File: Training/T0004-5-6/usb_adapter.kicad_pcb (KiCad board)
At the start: 2 copper layers, 50.8 x 25.4 mm, 23 parts, among them J1 modular8_rev3_comms_out, P1 USB_OTG, U1 FT231X, U2 TE_1825058-1

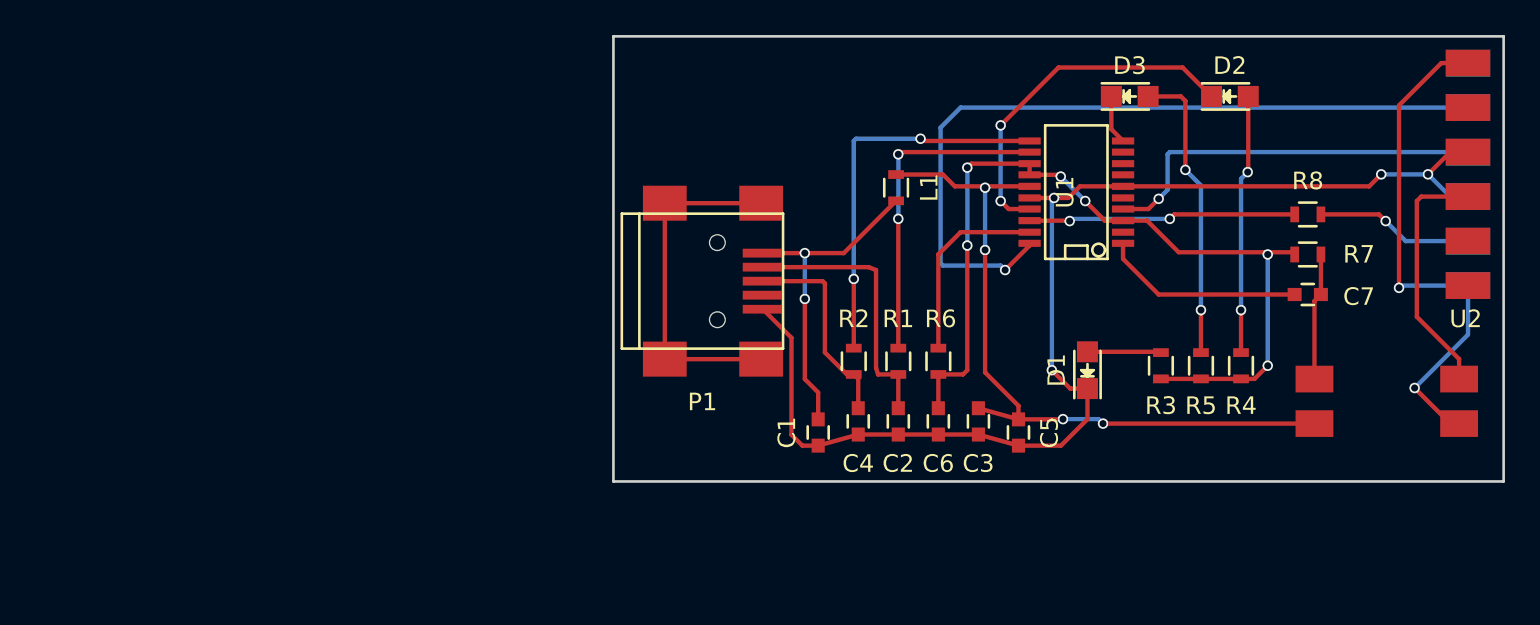
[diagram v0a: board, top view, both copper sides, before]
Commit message: generated gerbers
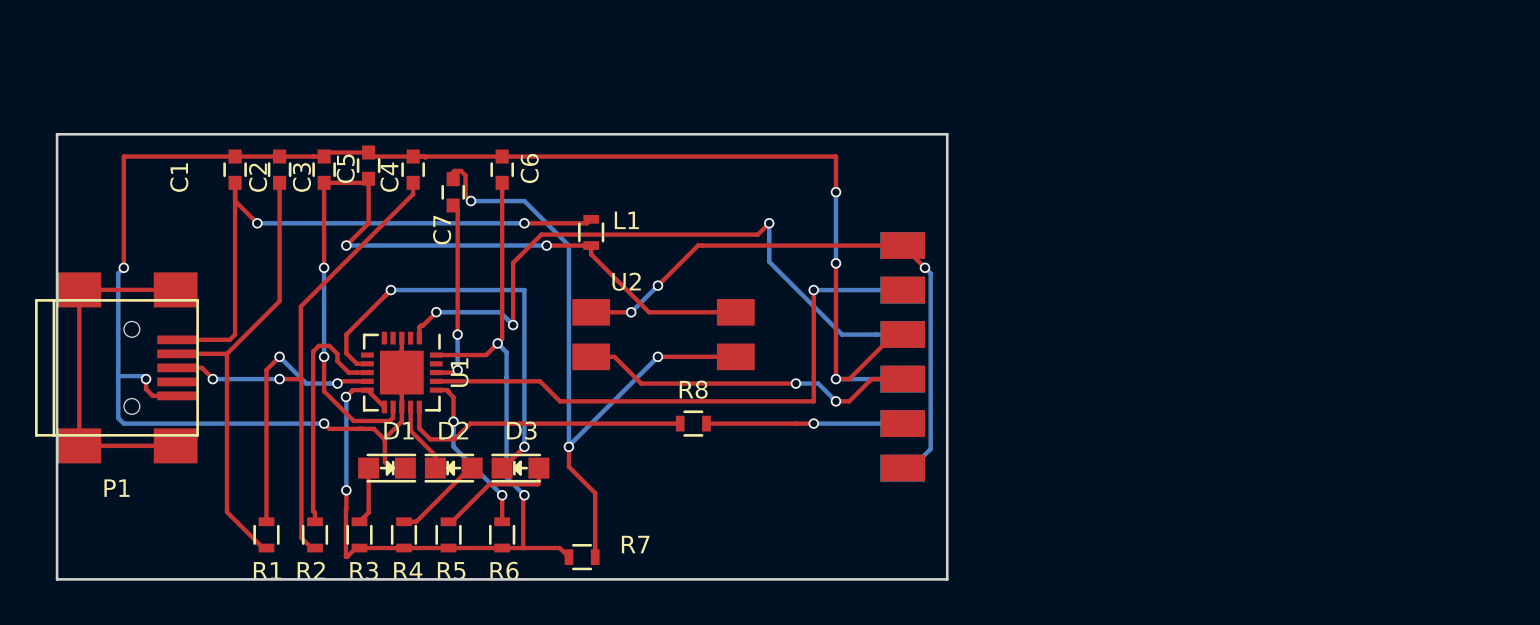
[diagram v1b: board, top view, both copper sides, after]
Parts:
- U1: value FT231X -> FT231XQ; footprint SMD_Packages:SSOP-20 -> Housings_DFN_QFN:QFN-20-1EP_4x4mm_Pitch0.5mm
- moved U2 49.9 mm to (141.0, 92.7), turned to 0 degrees
- moved C7 49.1 mm to (133.1, 85.9), turned to 90 degrees
- moved D2 49.1 mm to (133.1, 101.6)
- moved R4 48.7 mm to (130.3, 105.4)
- moved R3 46.7 mm to (127.8, 105.4)
- moved R7 44.9 mm to (140.4, 106.7)
- moved R5 44.0 mm to (132.8, 105.4)
- moved D3 40.7 mm to (136.9, 101.6)
- moved D1 40.4 mm to (129.3, 101.6), turned to 180 degrees
- moved C5 40.1 mm to (128.3, 84.3), turned to 90 degrees
- moved C3 40.0 mm to (125.7, 84.6), turned to 90 degrees
- moved U1 39.8 mm to (130.2, 96.1), turned to 270 degrees
- moved C2 38.1 mm to (123.2, 84.6), turned to 90 degrees
- moved R1 37.4 mm to (122.4, 105.4)
- moved R8 37.0 mm to (146.8, 99.1)
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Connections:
- U1 pad 1: Net-(C7-Pad1) -> /RX
- U1 pad 10: /~TXLED -> +3V3
- U1 pad 11: Net-(R2-Pad1) -> +3V3
- U1 pad 12: Net-(R1-Pad1) -> +5V
- U1 pad 13: +3V3 -> GND
- U1 pad 14: +3V3 -> /~RXLED
- U1 pad 15: +5V -> /TXDEN
- U1 pad 16: GND -> /~SLEEP
- U1 pad 17: /~RXLED -> /TX
- U1 pad 18: /TXDEN -> Net-(C7-Pad1)
- U1 pad 19: /~SLEEP -> Net-(U1-Pad19)
- U1 pad 20: /TX -> +3V3
- U1 pad 3: +3V3 -> GND
- U1 pad 4: /RX -> Net-(U1-Pad4)
- U1 pad 6: GND -> Net-(U1-Pad6)
- U1 pad 7: Net-(U1-Pad7) -> /~TXLED
- U1 pad 8: Net-(U1-Pad8) -> Net-(R2-Pad1)
- U1 pad 9: Net-(U1-Pad9) -> Net-(R1-Pad1)
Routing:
- net GND: track 68.8 -> 108.7 mm, vias 4 -> 6
- net /PROGRAM: track 7.26 -> 39.6 mm, vias 0 -> 3
- net /~TXLED: track 2.82 -> 24.9 mm, vias 0 -> 2
- net Net-(C4-Pad1): track 11.7 -> 31.3 mm, vias 0 -> 2
- net /~RXLED: track 20.2 -> 4.07 mm, vias 2 -> 0
- net Net-(C1-Pad1): track 18.6 -> 34.1 mm
- net /RX: track 22.2 -> 37.3 mm, vias 1 -> 3
- net /TX: track 44.3 -> 33.4 mm
- net Net-(C2-Pad1): track 15.5 -> 26.0 mm
- net Net-(D3-Pad2): track 17.0 -> 6.92 mm, vias 2 -> 0
- net Net-(D2-Pad2): track 14.8 -> 5.16 mm, vias 2 -> 0
- net Net-(R2-Pad1): track 22.0 -> 13.9 mm, vias 2 -> 0
- net +5V: track 41.5 -> 48.3 mm
- net Net-(J1-Pad7): track 14.2 -> 19.4 mm, vias 0 -> 2
- net /POWER_OUT: track 29.8 -> 33.7 mm, vias 2 -> 3
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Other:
- board text removed: "USB to serial Jeremy OpenRobotics.ca"
